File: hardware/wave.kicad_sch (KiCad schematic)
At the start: 62 parts, among them J101 WAGO 2065-100, J102 WAGO 2065-100, J103 Cortex, J104 WAGO 2065-100, J105 WAGO 2065-100, J106 WAGO 2065-100, J107 WAGO 2065-100, SW101 SKSG, SW102 SKSG, U101 ATSAMD51J, U102 TPS78433QWDRBRQ1, Y101 32k768

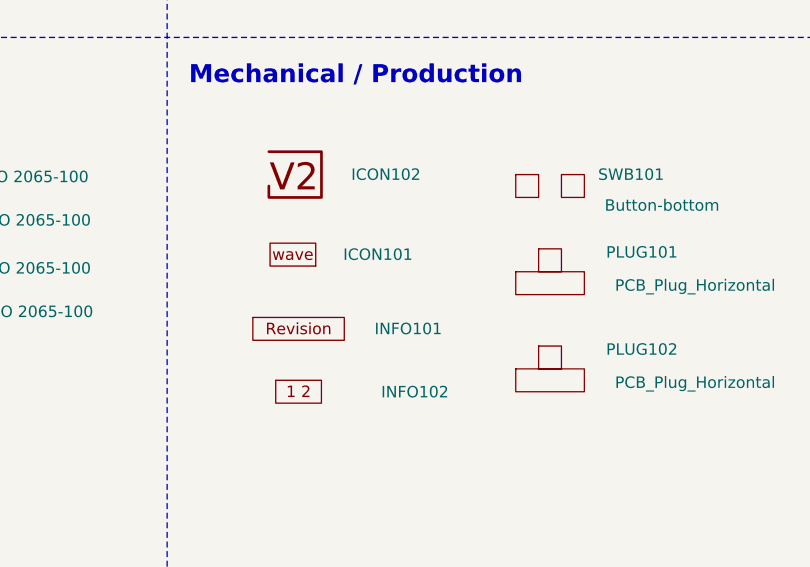
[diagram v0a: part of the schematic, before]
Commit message: Update stackup
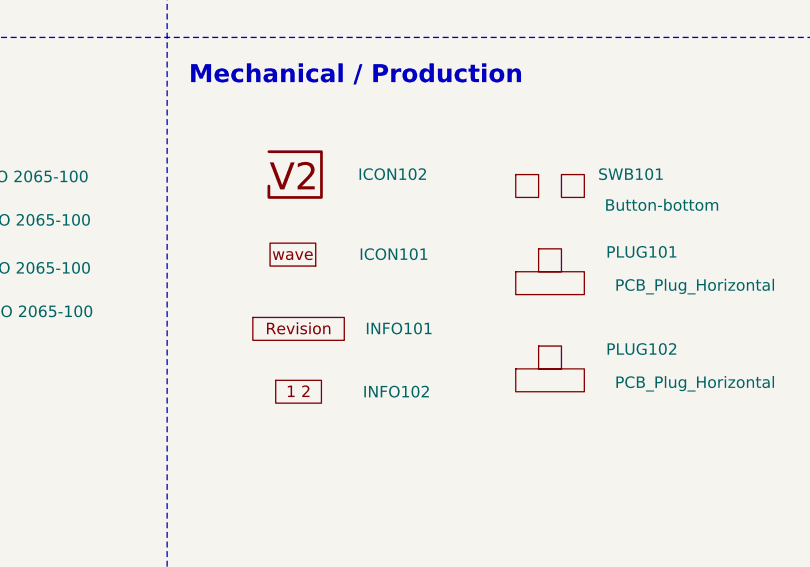
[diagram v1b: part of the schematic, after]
